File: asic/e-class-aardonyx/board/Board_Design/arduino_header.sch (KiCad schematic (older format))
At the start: 26 parts, among them J4 Conn_1x8, J5 Conn_1x6_F, J6 Conn_1x3_M, J7 Conn_1x10, J8 Conn_1x8, U13 MCP3008, U5 CAT24M01WI-GT3, U6 IS25LP256x-xM, U7 LSF0108PWR, U8 LSF0108PWR

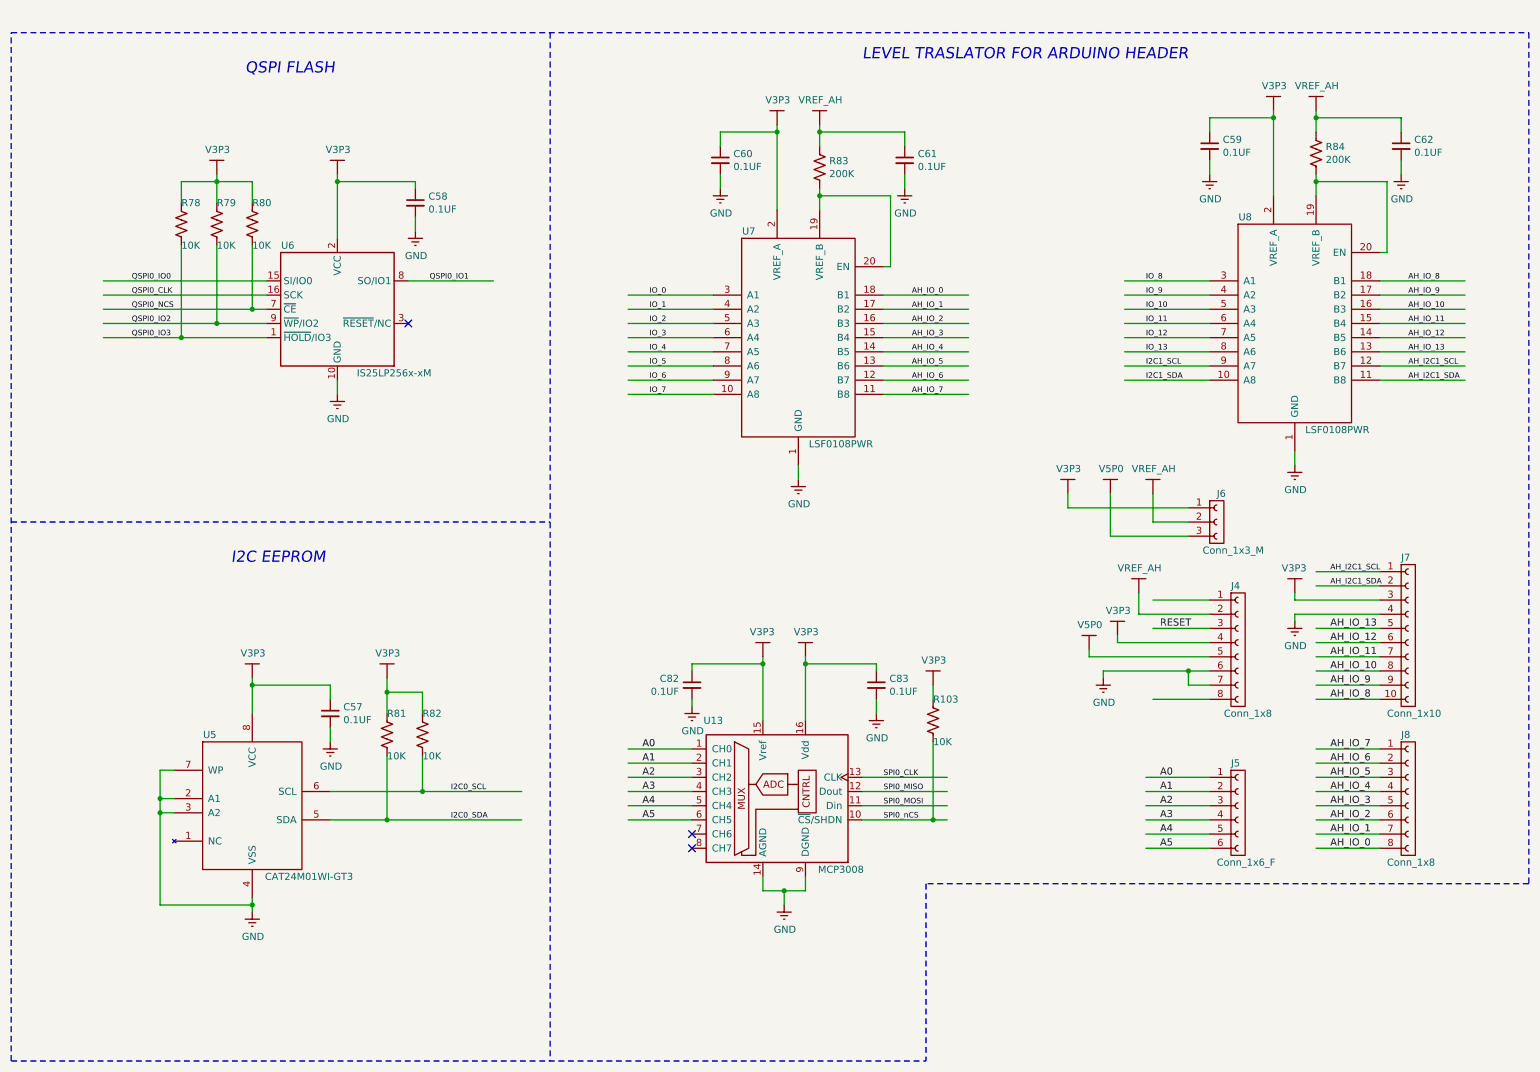
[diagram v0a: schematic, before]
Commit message: update
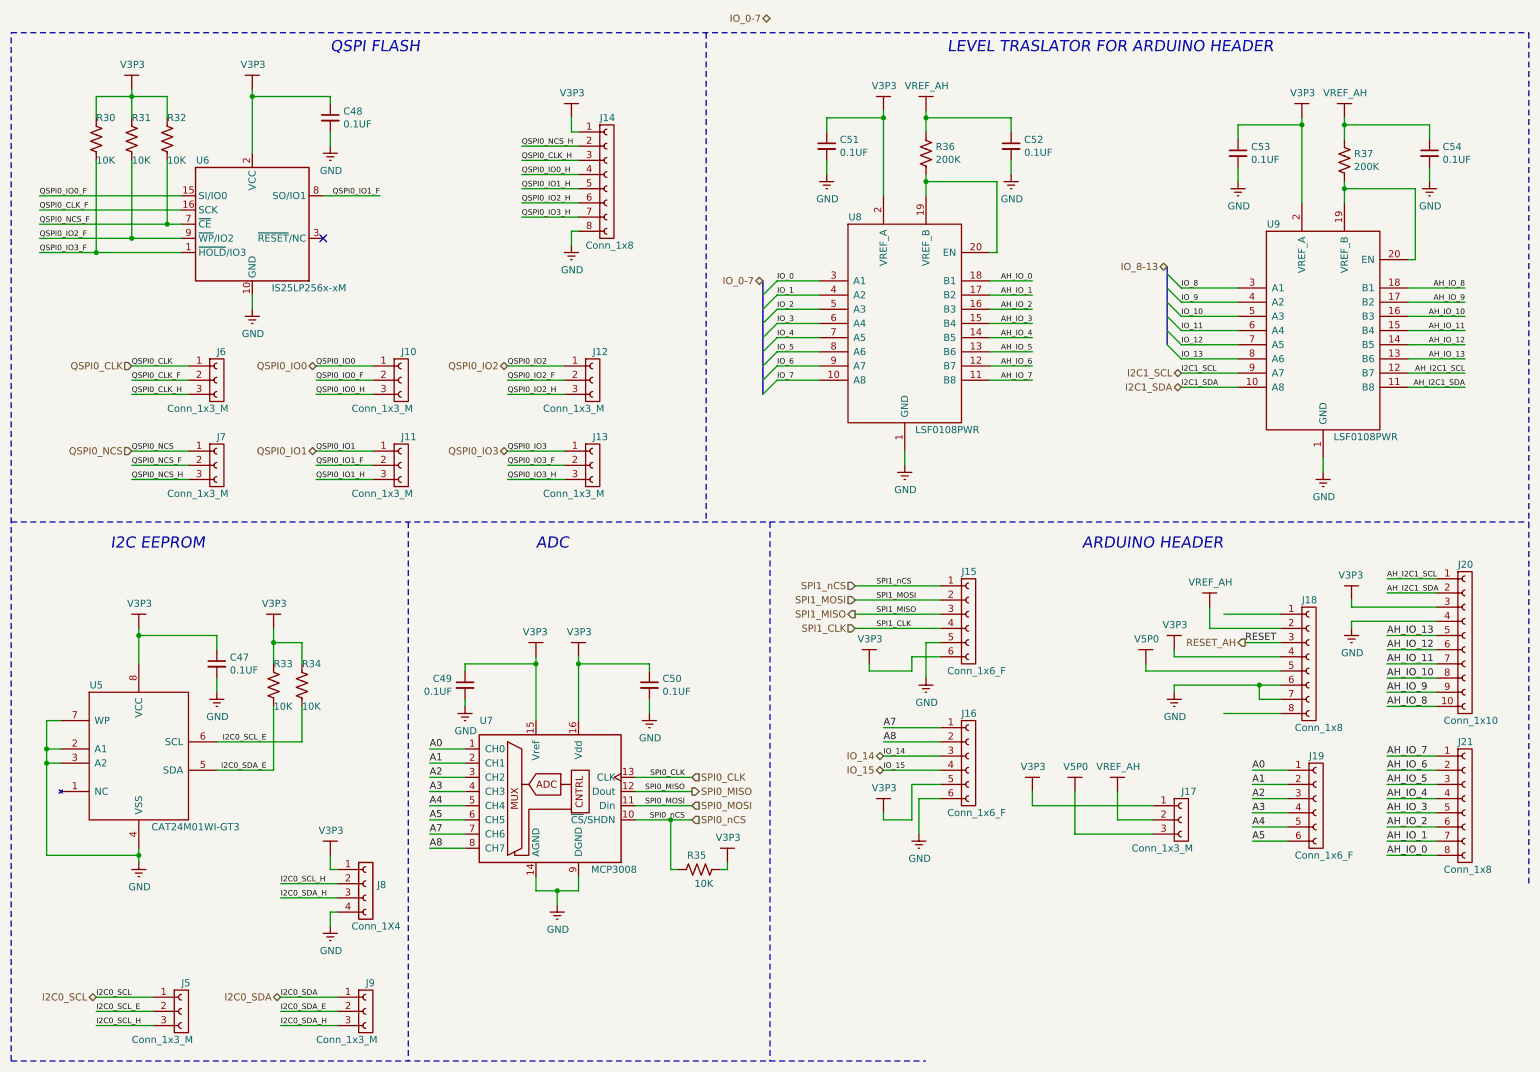
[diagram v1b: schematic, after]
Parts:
- added J10, J11, J12, J13, J5, J6, J7, J9: Conn_1x3_M, symbol aardonyx:Conn_1x3_M
- added J14: Conn_1x8, symbol aardonyx:Conn_1x8
- added J15, J16: Conn_1x6_F, symbol aardonyx:Conn_1x6_F
- added J8: Conn_1X4, symbol aardonyx:Conn_01x04
- renumbered C57 to C47, C58 to C48, C82 to C49, C83 to C50, C60 to C51, C61 to C52, C59 to C53, C62 to C54, J6 to J17, J4 to J18, J5 to J19, J7 to J20, J8 to J21, R78 to R30, R79 to R31, R80 to R32, R81 to R33, R82 to R34, R103 to R35, R83 to R36, R84 to R37, U13 to U7, U7 to U8, U8 to U9
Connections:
- net labels added: A7, A8, I2C0_SCL_E, I2C0_SCL_H, I2C0_SDA_E, I2C0_SDA_H, IO_0-7, IO_14, IO_15, IO_8-13, QSPI0_CLK_F, QSPI0_CLK_H, QSPI0_IO0_F, QSPI0_IO0_H, QSPI0_IO1_F, QSPI0_IO1_H, QSPI0_IO2_F, QSPI0_IO2_H, QSPI0_IO3_F, QSPI0_IO3_H, QSPI0_NCS_F, QSPI0_NCS_H, RESET_AH, SPI1_CLK, SPI1_MISO, SPI1_MOSI, SPI1_nCS
- wire segments 186 -> 248
- no-connect marks 3 -> 1
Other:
- note added: "ADC\n"
- note added: "ARDUINO HEADER\n"
- moved on the sheet: C47, C48, C49, C50, C51, C52, C53, C54, J17, J18, J19, J20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
